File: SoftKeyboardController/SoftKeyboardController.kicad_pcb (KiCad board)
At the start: 2 copper layers, 88.4 x 78.7 mm, 29 parts, among them IC1 PCA9956BTWY, J1 Barrel_Jack, J2 Conn_01x08_Socket, J3 Motor 1, J4 Motor 2, J5 Conn_01x12_Socket, J6 Conn_01x12_Socket, J7 EXT IMU Connection, J8 Conn_01x08_Socket, U1 Motor Driver DRV8847PWR, U2 ADC128D818, U3 ADC128D818, U4 PI4IOE5V9539LEX

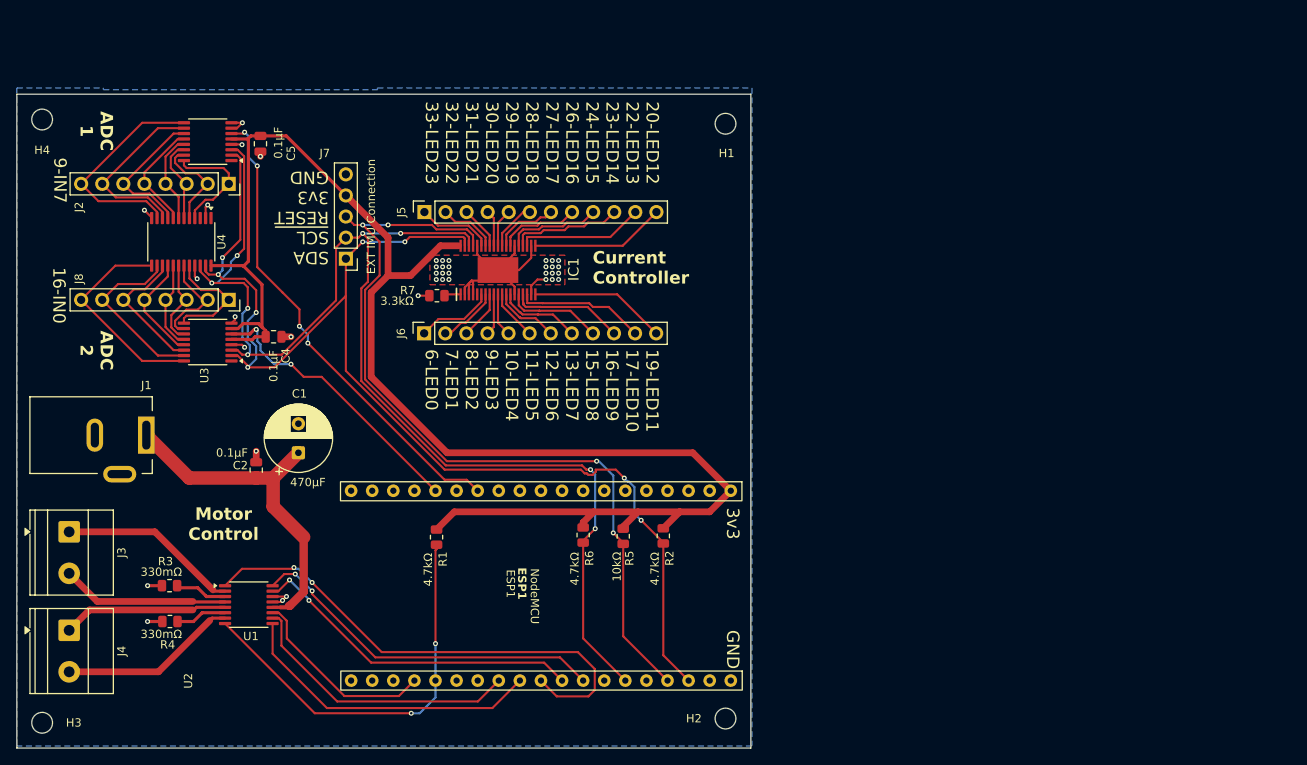
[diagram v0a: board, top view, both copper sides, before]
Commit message: Remapped Board again
Version of Board before ordering
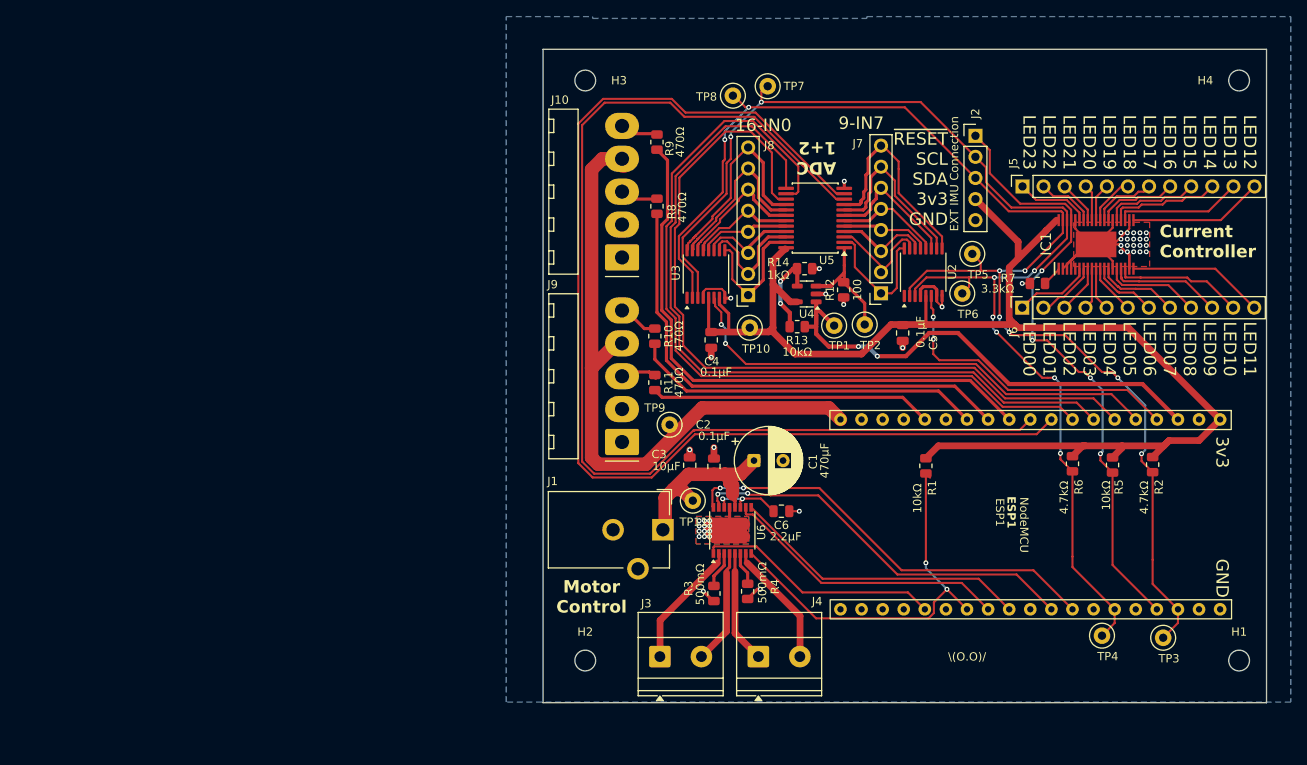
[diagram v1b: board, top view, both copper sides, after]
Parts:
- removed U1: Motor Driver DRV8847PWR, Package_SO:TSSOP-16_4.4x5mm_P0.65mm
- added C3: 10μF, Capacitor_SMD:C_0805_2012Metric, F.Cu at (170.1, 93.3)
- added C6: 2.2μF, Capacitor_SMD:C_0805_2012Metric, F.Cu at (181.1, 98.9)
- added J10: Motor Encoder 1, Connector_Molex:Molex_KK-396_A-41792-0005_1x05_P3.96mm_Horizontal, F.Cu at (161.9, 68.3)
- added J9: Motor Encoder 2, Connector_Molex:Molex_KK-396_A-41792-0005_1x05_P3.96mm_Horizontal, F.Cu at (161.9, 90.5)
- added R10: 470Ω, Resistor_SMD:R_0805_2012Metric, F.Cu at (165.9, 77.8)
- added R11: 470Ω, Resistor_SMD:R_0805_2012Metric, F.Cu at (165.9, 83.4)
- added R12: 100, Resistor_SMD:R_0805_2012Metric, F.Cu at (188.6, 72.2)
- added R13: 10kΩ, Resistor_SMD:R_0805_2012Metric, F.Cu at (183.0, 76.6)
- added R14: 1kΩ, Resistor_SMD:R_0805_2012Metric, F.Cu at (183.9, 69.6)
- added R8: 470Ω, Resistor_SMD:R_0805_2012Metric, F.Cu at (166.1, 62.1)
- added R9: 470Ω, Resistor_SMD:R_0805_2012Metric, F.Cu at (166.1, 54.4)
- added TP1: TestPoint, TestPoint:TestPoint_Loop_D1.80mm_Drill1.0mm_Beaded, F.Cu at (187.5, 76.5)
- added TP10: TestPoint, TestPoint:TestPoint_Loop_D1.80mm_Drill1.0mm_Beaded, F.Cu at (177.3, 76.8)
- added TP11: TestPoint, TestPoint:TestPoint_Loop_D1.80mm_Drill1.0mm_Beaded, F.Cu at (170.4, 97.6)
- added TP2: TestPoint, TestPoint:TestPoint_Loop_D1.80mm_Drill1.0mm_Beaded, F.Cu at (191.1, 76.4)
- added TP3: TestPoint, TestPoint:TestPoint_Loop_D1.80mm_Drill1.0mm_Beaded, F.Cu at (227.1, 114.1)
- added TP4: TestPoint, TestPoint:TestPoint_Loop_D1.80mm_Drill1.0mm_Beaded, F.Cu at (219.7, 113.8)
- added TP5: TestPoint, TestPoint:TestPoint_Loop_D1.80mm_Drill1.0mm_Beaded, F.Cu at (204.1, 67.9)
- added TP6: TestPoint, TestPoint:TestPoint_Loop_D1.80mm_Drill1.0mm_Beaded, F.Cu at (202.9, 72.6)
- added TP7: TestPoint, TestPoint:TestPoint_Loop_D1.80mm_Drill1.0mm_Beaded, F.Cu at (179.5, 47.7)
- added TP8: TestPoint, TestPoint:TestPoint_Loop_D1.80mm_Drill1.0mm_Beaded, F.Cu at (175.3, 48.8)
- added TP9: TestPoint, TestPoint:TestPoint_Loop_D1.80mm_Drill1.0mm_Beaded, F.Cu at (167.6, 88.4)
- added U5: CD74HC4067SM, Package_SO:SSOP-24_5.3x8.2mm_P0.65mm, F.Cu at (185.2, 63.6)
- added U6: DRV8848, Package_SO:TSSOP-16-1EP_4.4x5mm_P0.65mm, F.Cu at (175.2, 101.2)
- J1: value Barrel_Jack -> Barrel_Jack_Switch; footprint Connector_BarrelJack:BarrelJack_Kycon_KLDX-0202-xC_Horizontal -> Connector_BarrelJack:BarrelJack_CUI_PJ-102AH_Horizontal
- R1: value 4.7kΩ -> 10kΩ
- R3, R4: value 330mΩ -> 500mΩ
- U4: value PI4IOE5V9539LEX -> TL071; footprint Package_SO:TSSOP-24_4.4x7.8mm_P0.65mm -> Package_TO_SOT_SMD:SOT-23-5
- moved H4 144.2 mm to (236.2, 47.0)
- moved H3 101.3 mm to (157.5, 47.0)
- moved H1 89.5 mm to (236.2, 116.8)
- moved U2 87.6 mm to (198.2, 70.1), turned to 90 degrees
- moved J4 83.1 mm to (178.3, 116.4), turned to 0 degrees
- moved C5 80.6 mm to (195.7, 77.4)
- moved J7 79.6 mm to (193.1, 72.6), turned to 180 degrees
- moved J2 77.3 mm to (204.5, 53.6), turned to 0 degrees
- moved U4 75.6 mm to (184.2, 72.7), turned to 180 degrees
- moved J3 72.7 mm to (166.5, 116.4), turned to 0 degrees
- moved R7 72.3 mm to (211.9, 71.4)
- moved IC1 72.1 mm to (219.0, 66.7)
- moved J6 72.1 mm to (210.1, 74.3)
- moved J5 72.1 mm to (210.1, 59.7)
- moved R4 69.7 mm to (177.0, 108.5), turned to 90 degrees
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- renumbered J7 to J2, J2 to J7
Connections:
- ESP1 pad 10: unconnected-(ESP1-GPIO26/DAC2-Pad10) -> s0
- ESP1 pad 11: unconnected-(ESP1-GPIO27-Pad11) -> Net-(ESP1-GPIO27)
- ESP1 pad 12: unconnected-(ESP1-GPIO14-Pad12) -> Net-(ESP1-GPIO14)
- ESP1 pad 19: unconnected-(ESP1-Vin5V-Pad19) -> 5v
- ESP1 pad 23: Net-(ESP1-GPIO15) -> unconnected-(ESP1-GPIO15-Pad23)
- ESP1 pad 26: unconnected-(ESP1-GPIO4-Pad26) -> Net-(ESP1-GPIO4)
- ESP1 pad 29: Net-(ESP1-GPIO5) -> unconnected-(ESP1-GPIO5-Pad29)
- ESP1 pad 3: unconnected-(ESP1-GPIO36/ADC0-Pad3) -> I_Op
- ESP1 pad 4: unconnected-(ESP1-GPI39/ADC3-Pad4) -> Net-(ESP1-GPI39/ADC3)
- ESP1 pad 5: unconnected-(ESP1-GPI34/ADC6-Pad5) -> Net-(ESP1-GPI34/ADC6)
- ESP1 pad 6: unconnected-(ESP1-GPI35/ADC7-Pad6) -> ~{Multi}
- ESP1 pad 7: unconnected-(ESP1-GPIO32/ADC4-Pad7) -> s3
- ESP1 pad 8: unconnected-(ESP1-GPIO33/ADC5-Pad8) -> s2
- ESP1 pad 9: unconnected-(ESP1-GPIO25/DAC1-Pad9) -> s1
- J1 pad 3: (no net) -> unconnected-(J1-Pad3)
- J2 pad 1: SDA -> Net-(ESP1-GPIO1/TX0)
- J2 pad 3: Net-(ESP1-GPIO1/TX0) -> SDA
- J7 pad 1: Net-(J2-Pin_1) -> Net-(J7-Pin_1)
- J7 pad 2: Net-(J2-Pin_2) -> Net-(J7-Pin_2)
- J7 pad 3: Net-(J2-Pin_3) -> Net-(J7-Pin_3)
- J7 pad 4: Net-(J2-Pin_4) -> Net-(J7-Pin_4)
- J7 pad 5: Net-(J2-Pin_5) -> Net-(J7-Pin_5)
- J7 pad 6: Net-(J2-Pin_6) -> Net-(J7-Pin_6)
- J7 pad 7: Net-(J2-Pin_7) -> Net-(J7-Pin_7)
- J7 pad 8: Net-(J2-Pin_8) -> Net-(J7-Pin_8)
- R1 pad 2: Net-(ESP1-GPIO2) -> Net-(ESP1-GPIO4)
- U2 pad 10: Net-(J2-Pin_7) -> Net-(J7-Pin_7)
- U2 pad 11: Net-(J2-Pin_6) -> Net-(J7-Pin_6)
- U2 pad 12: Net-(J2-Pin_5) -> Net-(J7-Pin_5)
- U2 pad 13: Net-(J2-Pin_4) -> Net-(J7-Pin_4)
- U2 pad 14: Net-(J2-Pin_3) -> Net-(J7-Pin_3)
- U2 pad 15: Net-(J2-Pin_2) -> Net-(J7-Pin_2)
- U2 pad 16: Net-(J2-Pin_1) -> Net-(J7-Pin_1)
- U2 pad 6: Net-(ESP1-GPIO12) -> Net-(ESP1-GPI39/ADC3)
- U2 pad 9: Net-(J2-Pin_8) -> Net-(J7-Pin_8)
- U3 pad 6: Net-(ESP1-GPIO13) -> Net-(ESP1-GPI34/ADC6)
- U4 pad 1: unconnected-(U4-~{INT}-Pad1) -> I_Op
- U4 pad 3: unconnected-(U4-~{RESET}-Pad3) -> Net-(U4-+)
- U4 pad 4: Net-(J2-Pin_1) -> Net-(U4--)
- U4 pad 5: Net-(J2-Pin_2) -> +3V3
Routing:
- net s1: track 0.00 -> 139.4 mm
- net s0: track 0.00 -> 135.3 mm
- net ~{Multi}: track 0.00 -> 98.4 mm
- net s2: track 0.00 -> 98.0 mm
- net s3: track 0.00 -> 95.7 mm
- net 5v: track 0.00 -> 78.9 mm
- net Net-(ESP1-GPIO27): track 0.00 -> 70.2 mm
- net Net-(ESP1-GPIO5): track 60.6 -> 0.00 mm, vias 2 -> 0
- net Net-(ESP1-GPIO14): track 0.00 -> 59.8 mm
- net I_Op: track 0.00 -> 59.4 mm, vias 0 -> 2
- net Net-(ESP1-GPI34/ADC6): track 0.00 -> 59.4 mm, vias 0 -> 2
- net Net-(ESP1-GPIO4): track 0.00 -> 48.1 mm, vias 0 -> 2
- net Net-(ESP1-GPI39/ADC3): track 0.00 -> 37.3 mm, vias 0 -> 2
- net Net-(J2-Pin_8): track 26.7 -> 0.00 mm
- net Net-(J7-Pin_8): track 0.00 -> 25.5 mm
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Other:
- board size 88.4 x 78.7 mm -> 87.1 x 78.7 mm
- board text added: "ADC 1+2"
- board text added: "LED11 LED10 LED09 LED08 LED07 LED06 LED05 LED04 LED03 LED02 LED01 LED00"
- board text added: "LED12 LED13 LED14 LED15 LED16 LED17 LED18 LED19 LED20 LED21 LED22 LED23"
- board text added: "\(O.O)/"
- board text added: "~{RESET} SCL SDA 3v3 GND"
- board text removed: "19-LED11 17-LED10 16-LED9 15-LED8 13-LED7 12-LED6 11-LED5 10-LED4 9-LED3 8-LED2 7-LED1 6-LED0"
- board text removed: "20-LED12 22-LED13 23-LED14 24-LED15 26-LED16 27-LED17 28-LED18 29-LED19 30-LED20 31-LED21 32-LED22 33-LED23"
- board text removed: "ADC 1"
- board text removed: "ADC 2"
- board text removed: "SDA SCL ~{RESET} 3v3 GND"
